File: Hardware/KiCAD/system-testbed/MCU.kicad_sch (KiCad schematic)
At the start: 1 part, among them U5 ESP32-WROVER-E

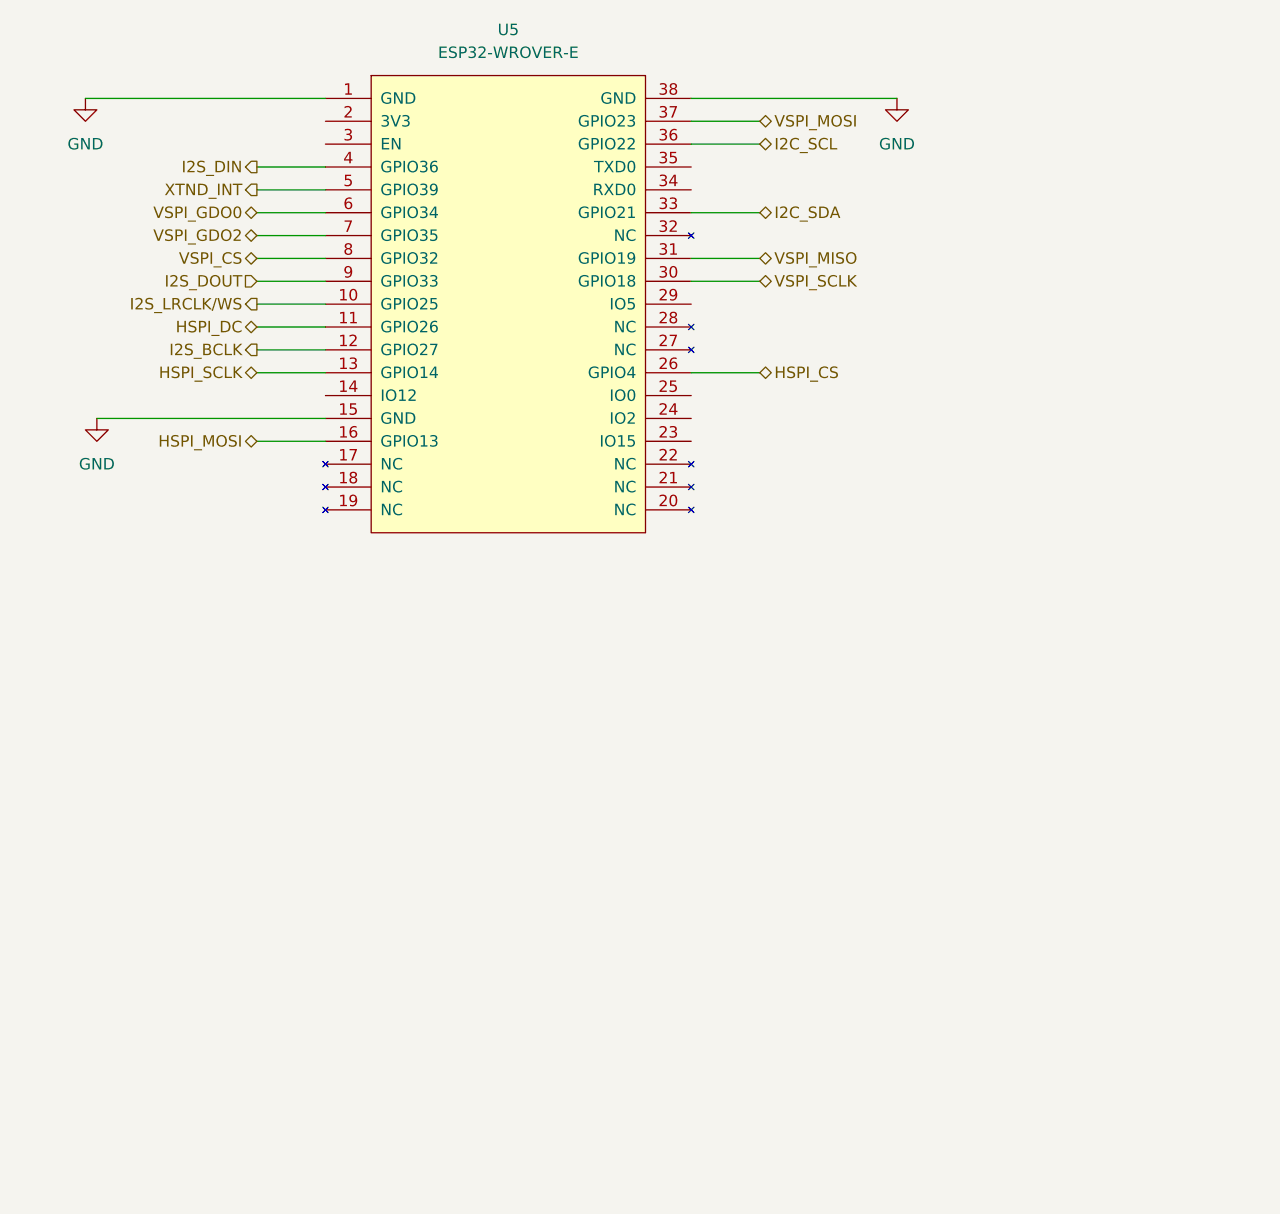
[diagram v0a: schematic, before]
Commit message: feat: schematic capture #63
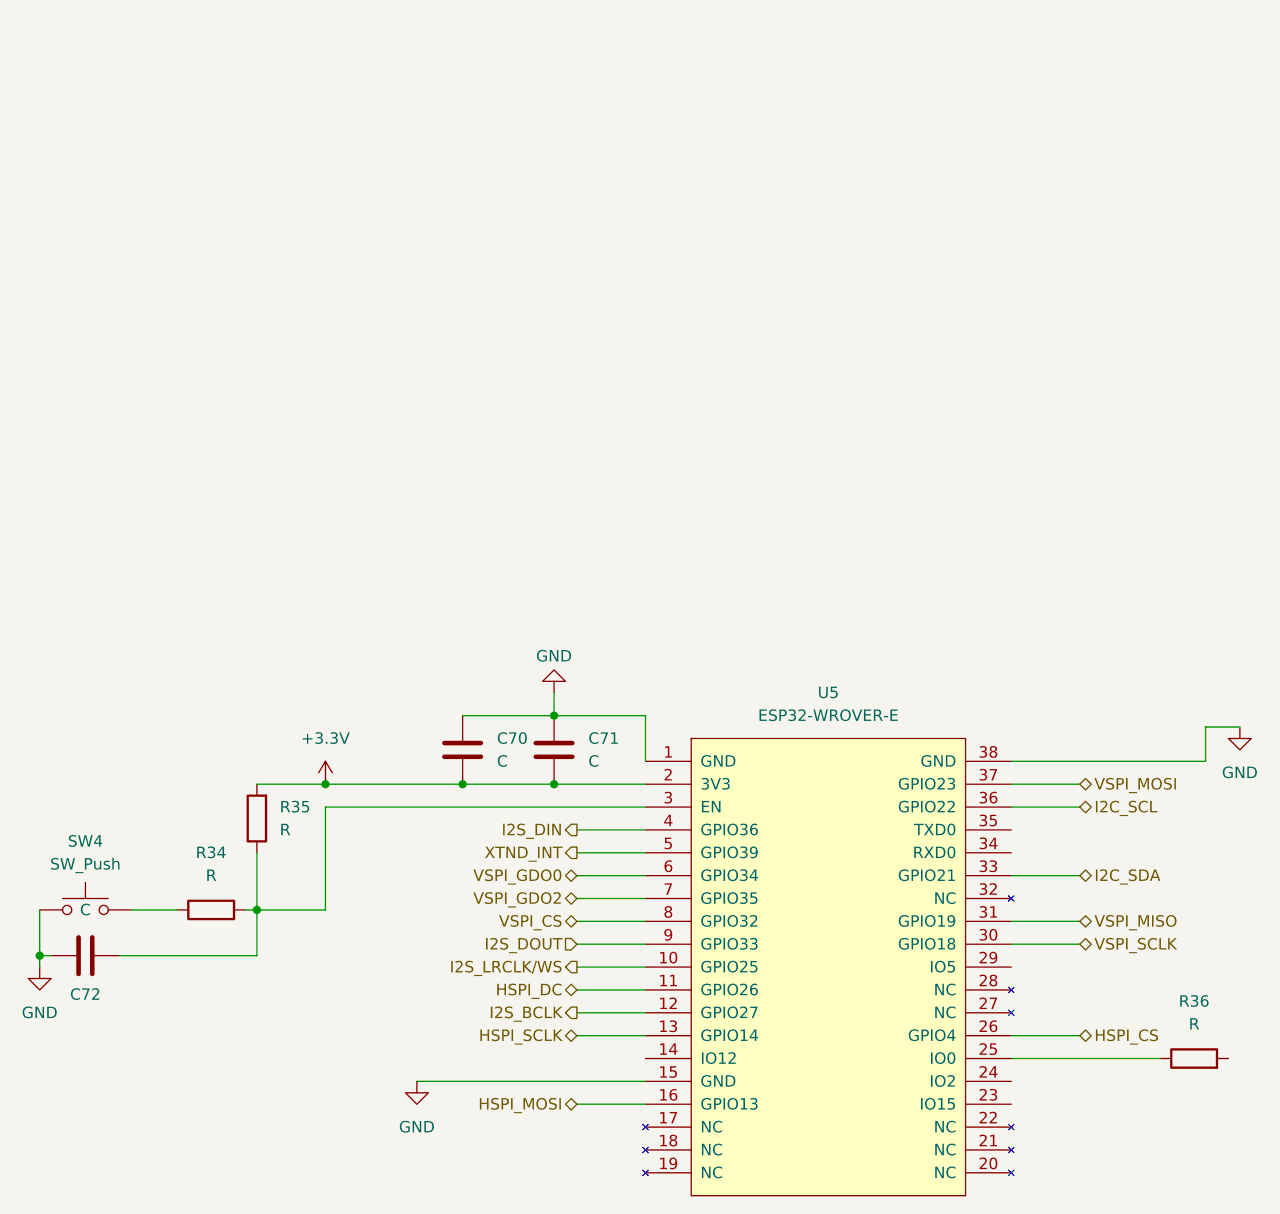
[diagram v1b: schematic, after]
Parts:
- added C70, C71, C72: C, symbol Device:C
- added R34, R35, R36: R, symbol Device:R
- added SW4: SW_Push, symbol Switch:SW_Push
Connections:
- net GND: now also C70.1, C71.1, C72.1, SW4.1
- net +3.3V: now reaches U5.2 (3V3)
- net +3.3V: now also C70.2, C71.2, R35.2
- net at U5.25 (IO0): now also R36.1
- net at U5.3 (EN): now also C72.2, R34.2, R35.1
- new net: R34.1, SW4.2
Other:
- moved on the sheet: U5
